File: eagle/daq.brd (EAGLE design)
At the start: 59.7 x 65.4 mm, 78 parts

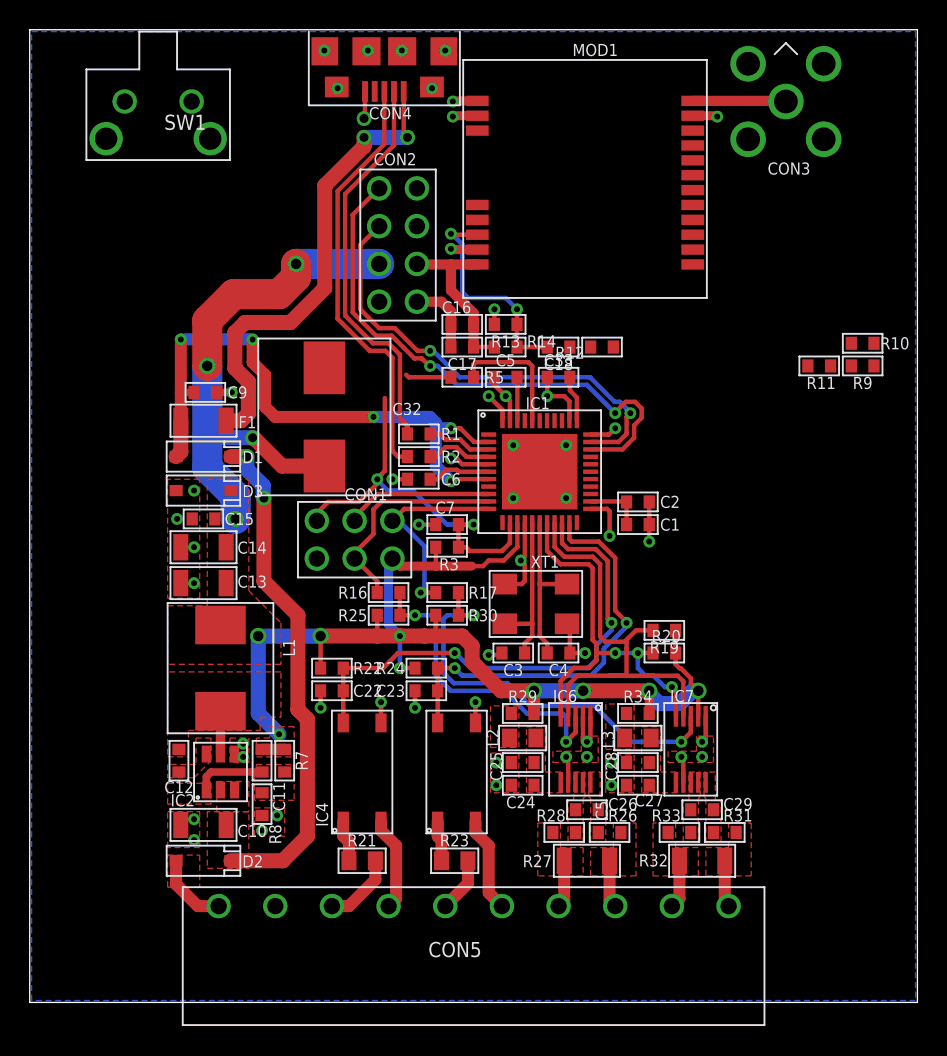
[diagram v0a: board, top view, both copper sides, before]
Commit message: do
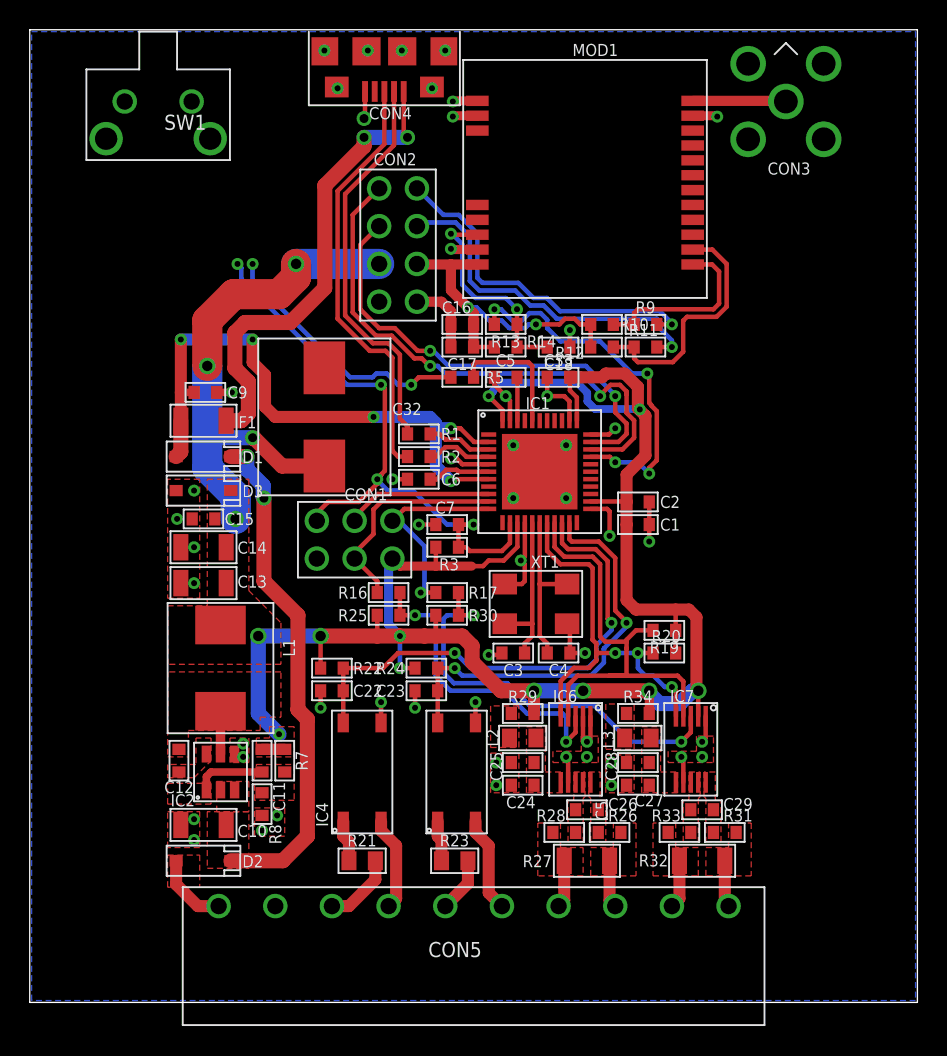
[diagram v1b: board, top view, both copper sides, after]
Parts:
- moved R10 17.6 mm to (38.5, 45.6)
- moved R9 14.9 mm to (41.4, 45.6), turned to 180 degrees
- moved R11 11.8 mm to (41.4, 44.1), turned to 180 degrees
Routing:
- net VCC: track 122.5 -> 161.1 mm, vias 14 -> 15
- net N$22: track 1.02 -> 25.4 mm, vias 1 -> 4
- net N$16: track 0.18 -> 24.0 mm, vias 0 -> 1
- net N$14: track 0.00 -> 23.7 mm, vias 0 -> 1
- net N$7: track 0.00 -> 16.8 mm
- net N$26: track 3.08 -> 17.7 mm, vias 0 -> 2
- net N$41: track 26.8 -> 41.3 mm, vias 2 -> 4
- net N$6: track 0.00 -> 12.3 mm
- net N$13: track 11.7 -> 22.4 mm, vias 0 -> 2
- net GND: track 73.6 -> 74.8 mm, vias 51 -> 52
